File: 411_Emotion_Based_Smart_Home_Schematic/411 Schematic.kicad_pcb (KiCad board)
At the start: 2 copper layers, 110 x 40 mm, 8 parts, among them Q1 NSS1C301ET4G, Q2 NSS1C301ET4G, Q3 NSS1C301ET4G, U4 HC-SR04

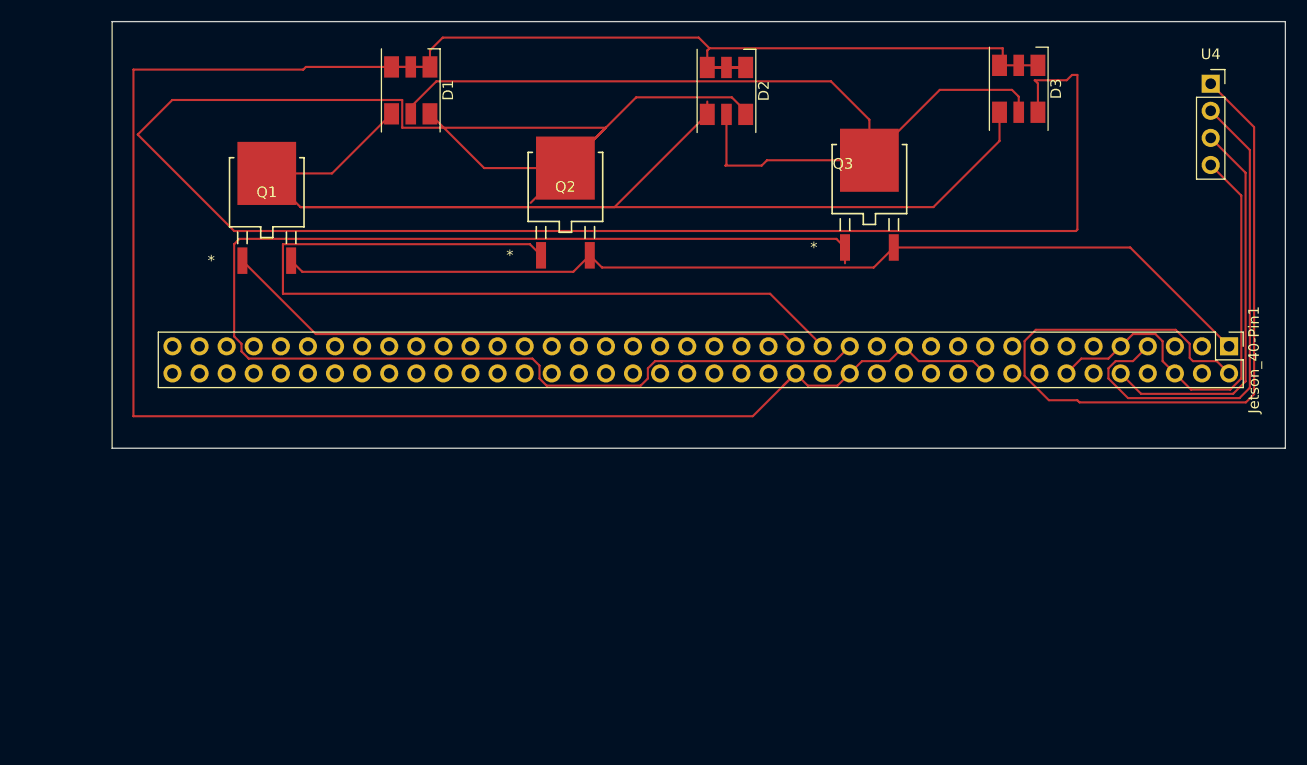
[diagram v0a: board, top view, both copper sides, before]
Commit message: Updated schematic.
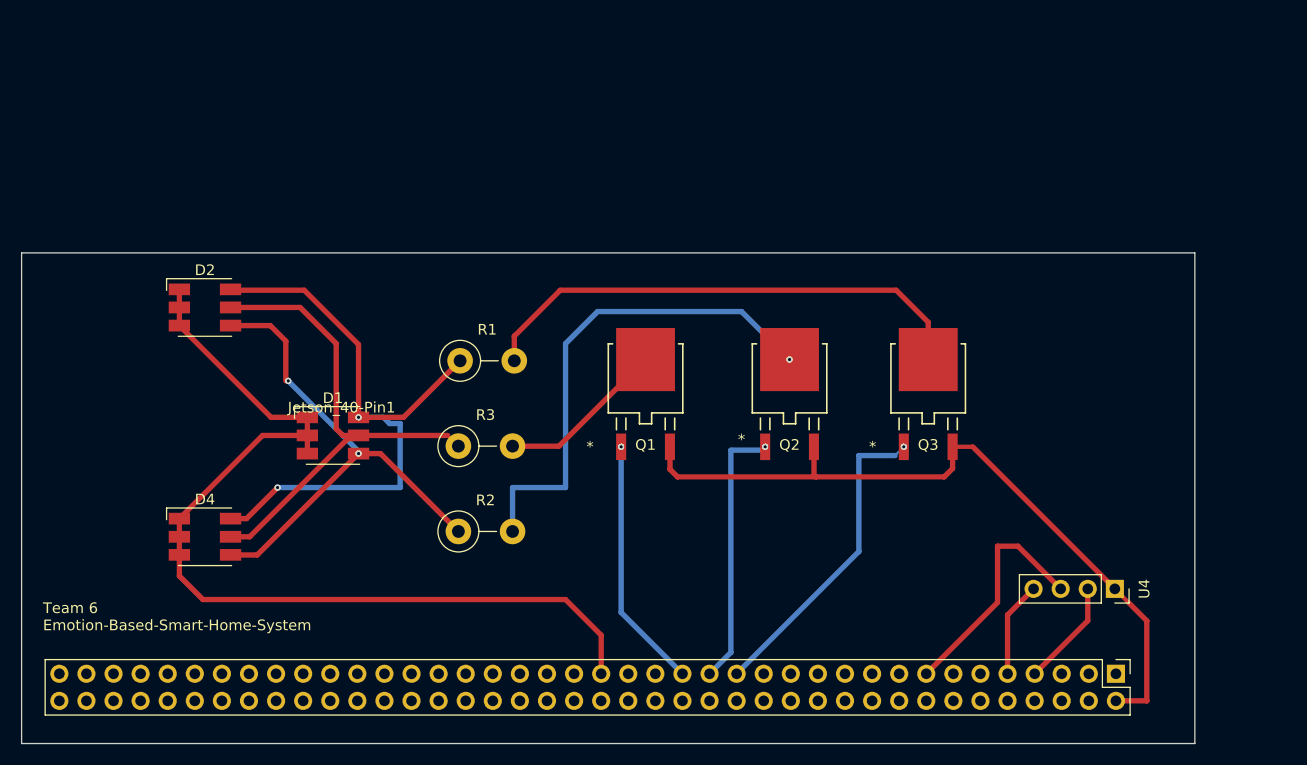
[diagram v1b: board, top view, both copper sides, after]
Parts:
- removed D3: Inolux_IN-P55TATRGB, LED_SMD:LED_Inolux_IN-P55TATRGB_PLCC6_5.0x5.5mm_P1.8mm
- added D4: LED_RGB, LED_SMD:LED_RGB_5050-6, F.Cu at (62.7, 80.6)
- added R1: 10, Resistor_THT:R_Axial_DIN0411_L9.9mm_D3.6mm_P5.08mm_Vertical, F.Cu at (86.6, 64.1)
- added R2: 10, Resistor_THT:R_Axial_DIN0411_L9.9mm_D3.6mm_P5.08mm_Vertical, F.Cu at (86.5, 80.1)
- added R3: 10, Resistor_THT:R_Axial_DIN0411_L9.9mm_D3.6mm_P5.08mm_Vertical, F.Cu at (86.5, 72.1)
- D1, D2: value Inolux_IN-P55TATRGB -> LED_RGB; footprint LED_SMD:LED_Inolux_IN-P55TATRGB_PLCC6_5.0x5.5mm_P1.8mm -> LED_SMD:LED_RGB_5050-6
- Q1, Q2, Q3: footprint Transistor411Library:DPAK-4_6P22X6P73_ONS -> NSS1C301ET4G:DPAK-4_6P22X6P73_ONS
- moved D2 52.9 mm to (62.7, 59.1), turned to 0 degrees
- moved U4 48.2 mm to (148.0, 85.5), turned to -90 degrees
- moved Q1 39.6 mm to (104.0, 65.8)
- moved D1 33.2 mm to (74.7, 71.1), turned to 0 degrees
- moved Jetson_40-Pin1 32.5 mm to (148.1, 93.5)
- moved Q2 27.6 mm to (117.5, 65.8)
- moved Q3 19.5 mm to (130.5, 65.8)
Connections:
- D1 pad 4: Q1 -> Q2
- D1 pad 5: Q3 -> Q1
- D1 pad 6: Q2 -> Q3
- D2 pad 4: Q1 -> Q2
- D2 pad 5: Q3 -> Q1
- D2 pad 6: Q2 -> Q3
- Jetson_40-Pin1 pad 1: Net-(Q1-C) -> unconnected-(Jetson_40-Pin1-3.3V-Pad1)
- Jetson_40-Pin1 pad 10: Net-(Jetson_40-Pin1-UART1_RXD) -> unconnected-(Jetson_40-Pin1-UART1_RXD-Pad10)
- Jetson_40-Pin1 pad 14: GND -> unconnected-(Jetson_40-Pin1-GND-Pad14)
- Jetson_40-Pin1 pad 15: unconnected-(Jetson_40-Pin1-GPIO12-Pad15) -> Net-(Jetson_40-Pin1-GPIO12)
- Jetson_40-Pin1 pad 20: GND -> unconnected-(Jetson_40-Pin1-GND-Pad20)
- Jetson_40-Pin1 pad 25: GND -> unconnected-(Jetson_40-Pin1-GND-Pad25)
- Jetson_40-Pin1 pad 30: GND -> unconnected-(Jetson_40-Pin1-GND-Pad30)
- Jetson_40-Pin1 pad 34: GND -> unconnected-(Jetson_40-Pin1-GND-Pad34)
- Jetson_40-Pin1 pad 6: GND -> unconnected-(Jetson_40-Pin1-GND-Pad6)
- Jetson_40-Pin1 pad 9: GND -> Net-(U4-GND)
- Q1 pad 2: Net-(Q1-C) -> /5V
- Q1 pad 3: Q1 -> Net-(Q1-E)
- Q2 pad 2: Net-(Q1-C) -> /5V
- Q2 pad 3: Q2 -> Net-(Q2-E)
- Q3 pad 2: Net-(Q1-C) -> /5V
- Q3 pad 3: Q3 -> Net-(Q3-E)
- U4 pad 3: Net-(Jetson_40-Pin1-UART1_RXD) -> Net-(Jetson_40-Pin1-GPIO12)
- U4 pad 4: GND -> Net-(U4-GND)
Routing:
- net GND: track 264.2 -> 88.9 mm
- net Q2: track 207.4 -> 47.6 mm, vias 0 -> 2
- net Net-(Jetson_40-Pin1-GPIO01): track 129.8 -> 29.8 mm, vias 0 -> 1
- net Net-(Q1-C): track 94.1 -> 0.00 mm
- net Q1: track 132.9 -> 47.9 mm
- net Net-(Jetson_40-Pin1-GPIO11): track 81.9 -> 25.1 mm, vias 0 -> 1
- net Net-(Q3-E): track 0.00 -> 47.6 mm
- net Net-(Q2-E): track 0.00 -> 46.7 mm, vias 0 -> 1
- net /Ultrasonic Trigger: track 47.4 -> 10.0 mm
- net Net-(Jetson_40-Pin1-UART1_RXD): track 37.2 -> 0.00 mm
- net Net-(Jetson_40-Pin1-GPIO13): track 55.2 -> 23.7 mm, vias 0 -> 1
- net Q3: track 90.5 -> 59.9 mm, vias 0 -> 2
- net Net-(Jetson_40-Pin1-GPIO12): track 0.00 -> 22.3 mm
- net Net-(Q1-E): track 0.00 -> 15.8 mm
- net /5V: track 79.0 -> 69.5 mm
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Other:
- board size 110 x 40 mm -> 110 x 46 mm
- board text added: "Team 6 Emotion-Based-Smart-Home-System"
